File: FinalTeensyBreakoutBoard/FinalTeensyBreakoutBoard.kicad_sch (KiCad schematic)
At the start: 31 parts, among them J1 POWER, J2 MC1, J3 MC2, J4 MC3, J5 CurrSB, J6 UWB1, J7 UWBchip, U1 Teensy4.1, U2 MAX3284E, U3 MAX3284E, U4 MAX3284E, U5 MAX3284E, U6 MAX3284E, U7 MAX3284E

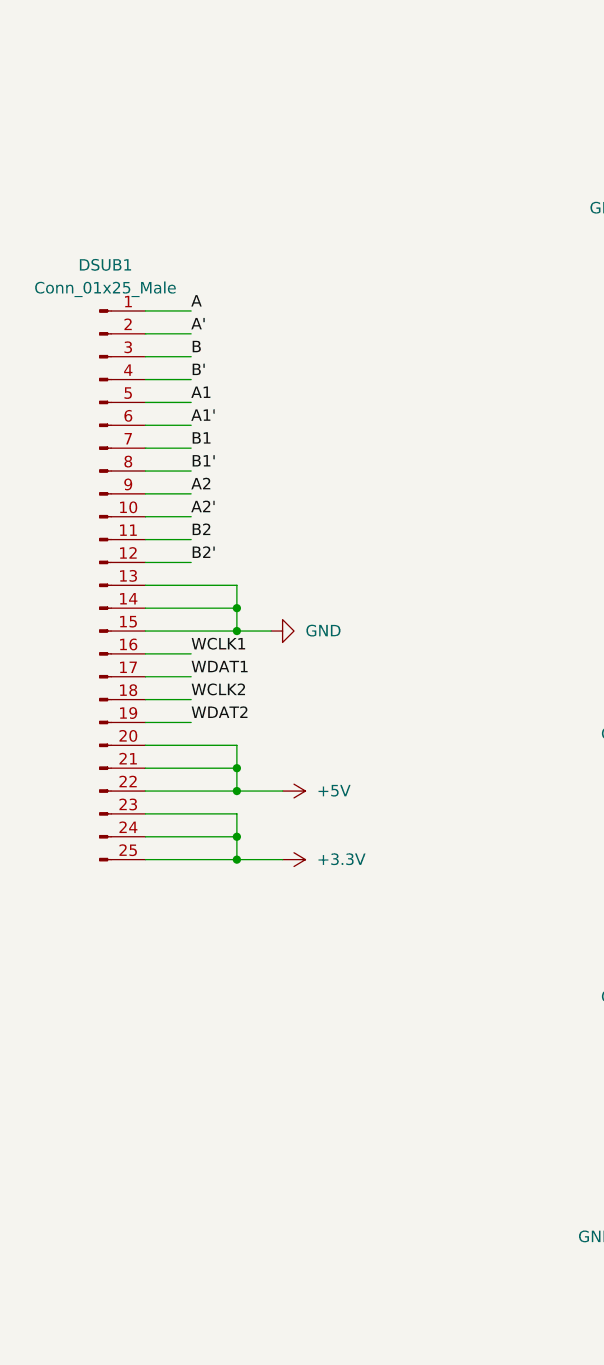
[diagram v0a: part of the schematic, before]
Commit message: Add files via upload
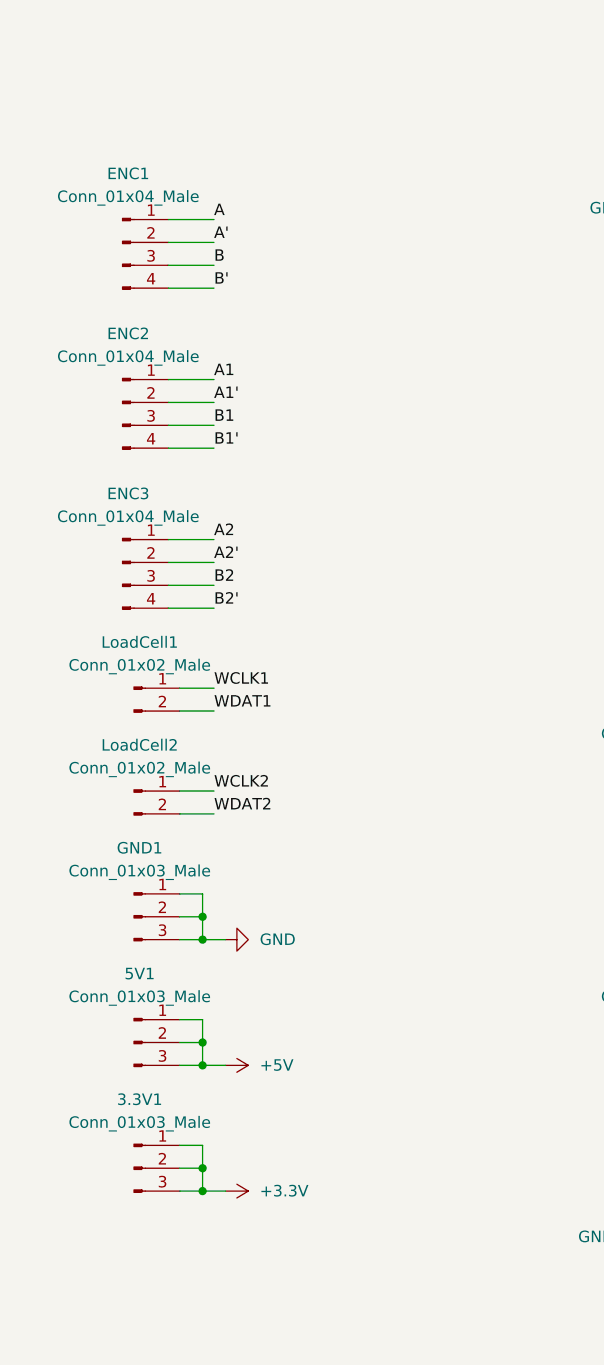
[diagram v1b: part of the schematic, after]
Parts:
- removed DSUB1: Conn_01x25_Male, Resistor_THT:R_Axial_DIN0207_L6.3mm_D2.5mm_P10.16mm_Horizontal, symbol Connector:Conn_01x25_Male
- added 3.3V1, 5V1, GND1: Conn_01x03_Male, teensy:3pinJST, symbol Connector:Conn_01x03_Male
- added ENC1, ENC2, ENC3: Conn_01x04_Male, teensy:4pinJST, symbol Connector:Conn_01x04_Male
- added LoadCell1, LoadCell2: Conn_01x02_Male, teensy:2pinJST, symbol Connector:Conn_01x02_Male
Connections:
- net +3.3V: now also 3.3V1.1 (Pin_1), 3.3V1.2 (Pin_2), 3.3V1.3 (Pin_3)
- net +5V: now also 5V1.1 (Pin_1), 5V1.2 (Pin_2), 5V1.3 (Pin_3)
- net A: now also ENC1.1 (Pin_1)
- net A': now also ENC1.2 (Pin_2)
- net A1: now also ENC2.1 (Pin_1)
- net A1': now also ENC2.2 (Pin_2)
- net A2: now also ENC3.1 (Pin_1)
- net A2': now also ENC3.2 (Pin_2)
- net B: now also ENC1.3 (Pin_3)
- net B': now also ENC1.4 (Pin_4)
- net B1: now also ENC2.3 (Pin_3)
- net B1': now also ENC2.4 (Pin_4)
- net B2: now also ENC3.3 (Pin_3)
- net B2': now also ENC3.4 (Pin_4)
- net GND: now also GND1.1 (Pin_1), GND1.2 (Pin_2), GND1.3 (Pin_3)
- net WCLK1: now also LoadCell1.1 (Pin_1)
- net WCLK2: now also LoadCell2.1 (Pin_1)
- net WDAT1: now also LoadCell1.2 (Pin_2)
- net WDAT2: now also LoadCell2.2 (Pin_2)
